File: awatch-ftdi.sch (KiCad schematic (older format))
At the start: 43 parts, among them J801 Molex 1050170001, J802 Conn_01x06, U801 AT93C46DN-SH-T, U802 MCP1703A-3302_SOT223, U803 FT2232HL, Y801 FH1200004

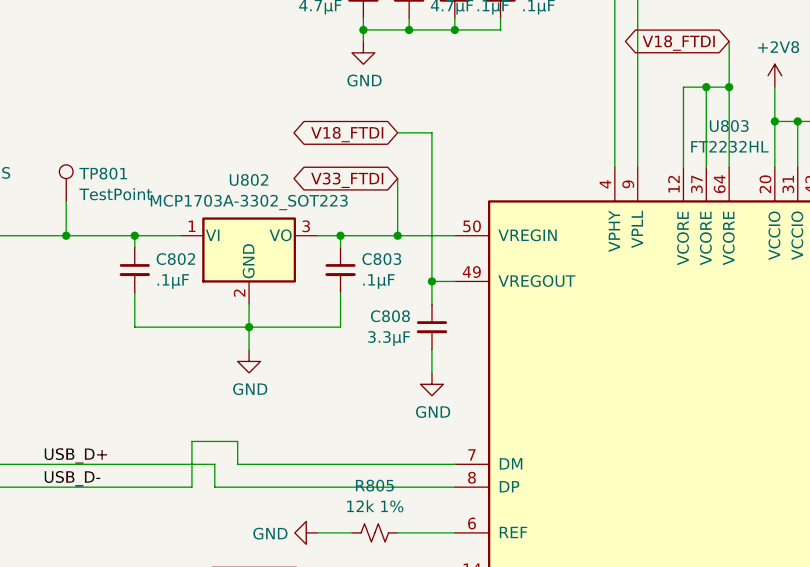
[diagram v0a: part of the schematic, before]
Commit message: Route FTDI.
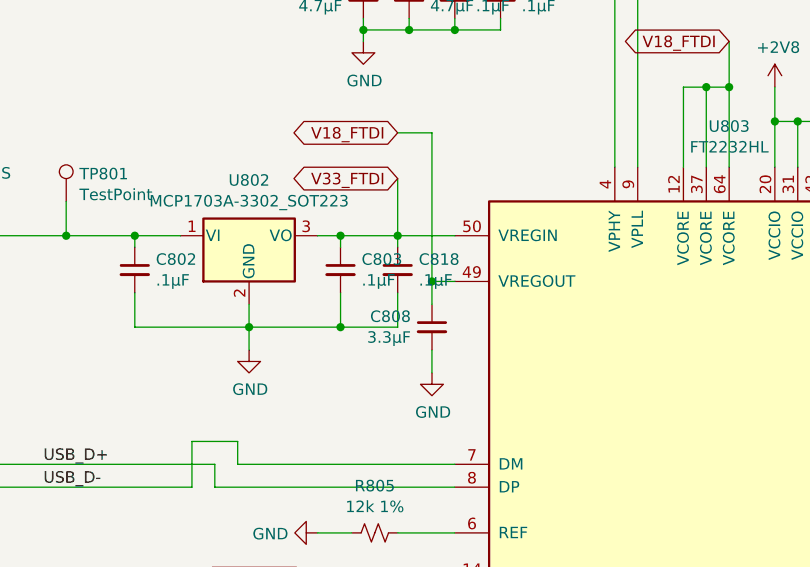
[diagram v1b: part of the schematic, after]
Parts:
- added C818: .1µF, Capacitor_SMD:C_0603_1608Metric, symbol Device:C_Small
- J802: footprint Connector_PinSocket_2.54mm:PinSocket_1x06_P2.54mm_Vertical -> Connector_PinHeader_2.54mm:PinHeader_1x06_P2.54mm_Vertical
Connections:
- net GND: now also C818.2
- net V33_FTDI: now also C818.1
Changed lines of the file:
@@
 F 0 "J802" H 10280 2792 50  0000 L CNN
 F 1 "Conn_01x06" H 10280 2701 50  0000 L CNN
-F 2 "Connector_PinSocket_2.54mm:PinSocket_1x06_P2.54mm_Vertical" H 10200 2800 50  0001 C CNN
+F 2 "Connector_PinHeader_2.54mm:PinHeader_1x06_P2.54mm_Vertical" H 10200 2800 50  0001 C CNN
 F 3 "~" H 10200 2800 50  0001 C CNN
 	1    10200 2800
@@
 Wire Wire Line
 	2500 3350 2500 2550
-Wire Wire Line
-	2500 2550 2850 2550
 Connection ~ 3150 2550
 $Comp
@@
 	2850 2400 2850 2550
 Connection ~ 2850 2550
-Wire Wire Line
-	2850 2550 3150 2550
 $Comp
 L Device:C_Small C804
@@
 Text Label 2650 5450 0    50   ~ 0
 DO
+Wire Wire Line
+	2850 2550 3150 2550
+Wire Wire Line
+	2500 2550 2850 2550
+$Comp
+L Device:C_Small C818
+U 1 1 5C2F6C15
+P 4300 2700
+F 0 "C818" H 4392 2746 50  0000 L CNN
+F 1 ".1µF" H 4392 2655 50  0000 L CNN
+F 2 "Capacitor_SMD:C_0603_1608Metric" H 4300 2700 50  0001 C CNN
+F 3 "~" H 4300 2700 50  0001 C CNN
+	1    4300 2700
+	1    0    0    -1
+$EndComp
+Wire Wire Line
+	4300 2550 4300 2600
+Wire Wire Line
+	4300 2800 4300 2950
+Wire Wire Line
+	4300 2950 4050 2950
+Connection ~ 4050 2950
 $EndSCHEMATC

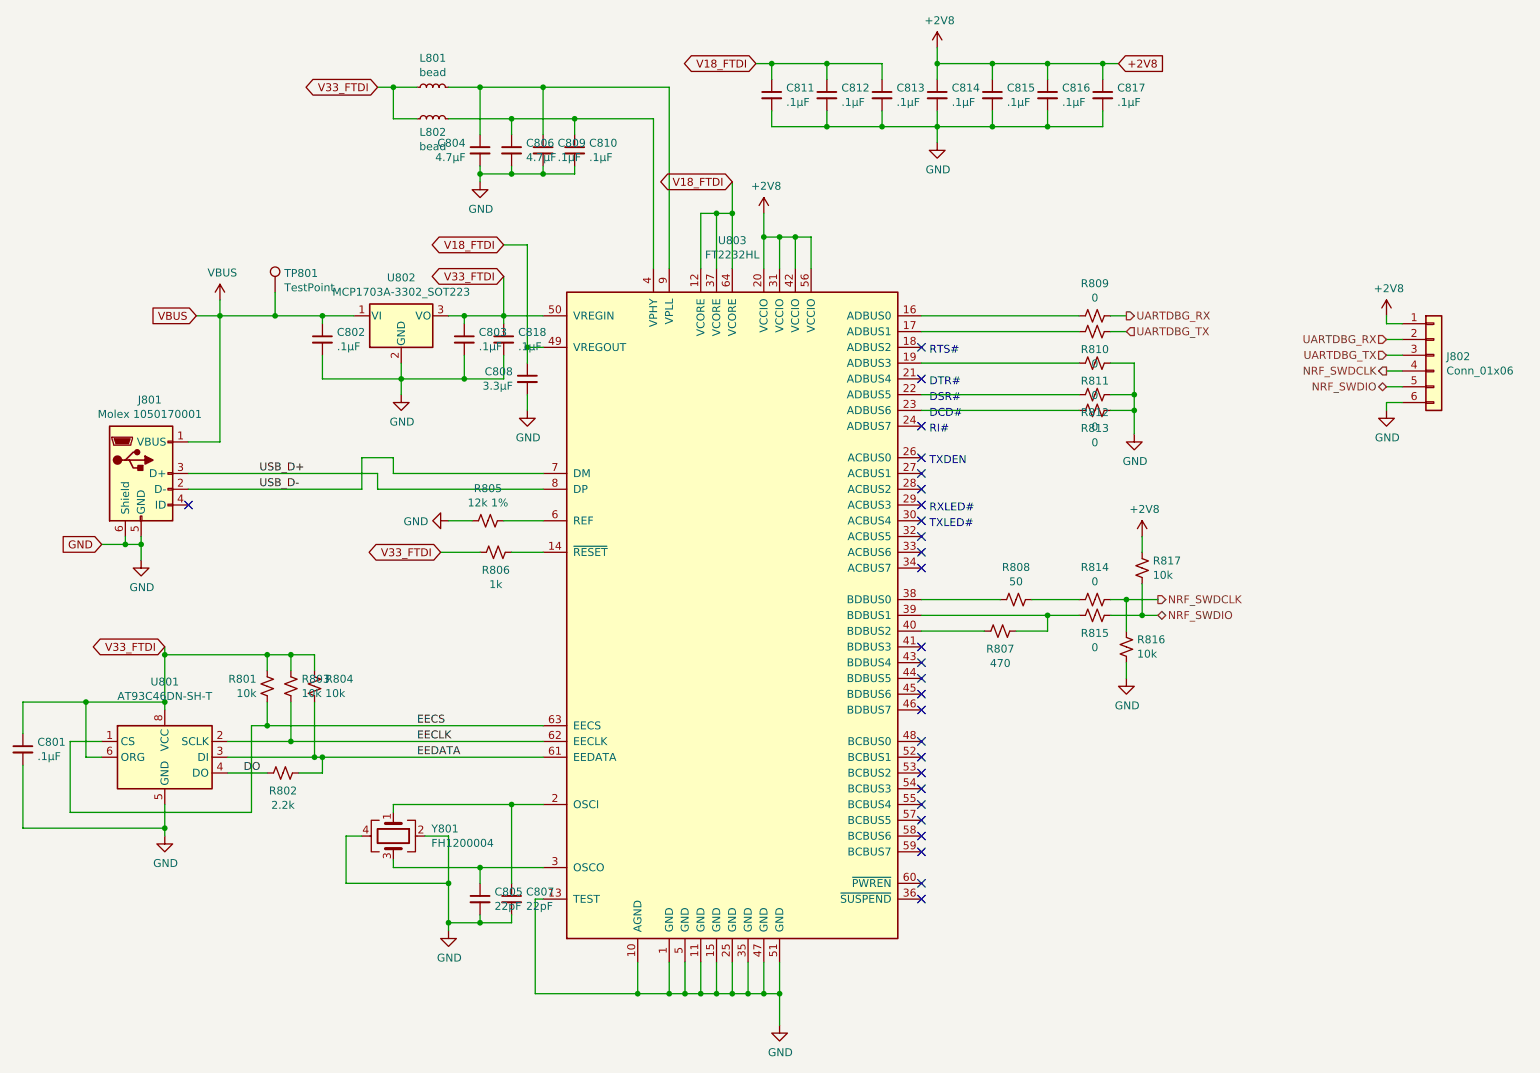
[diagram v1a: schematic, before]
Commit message: approx. final layout
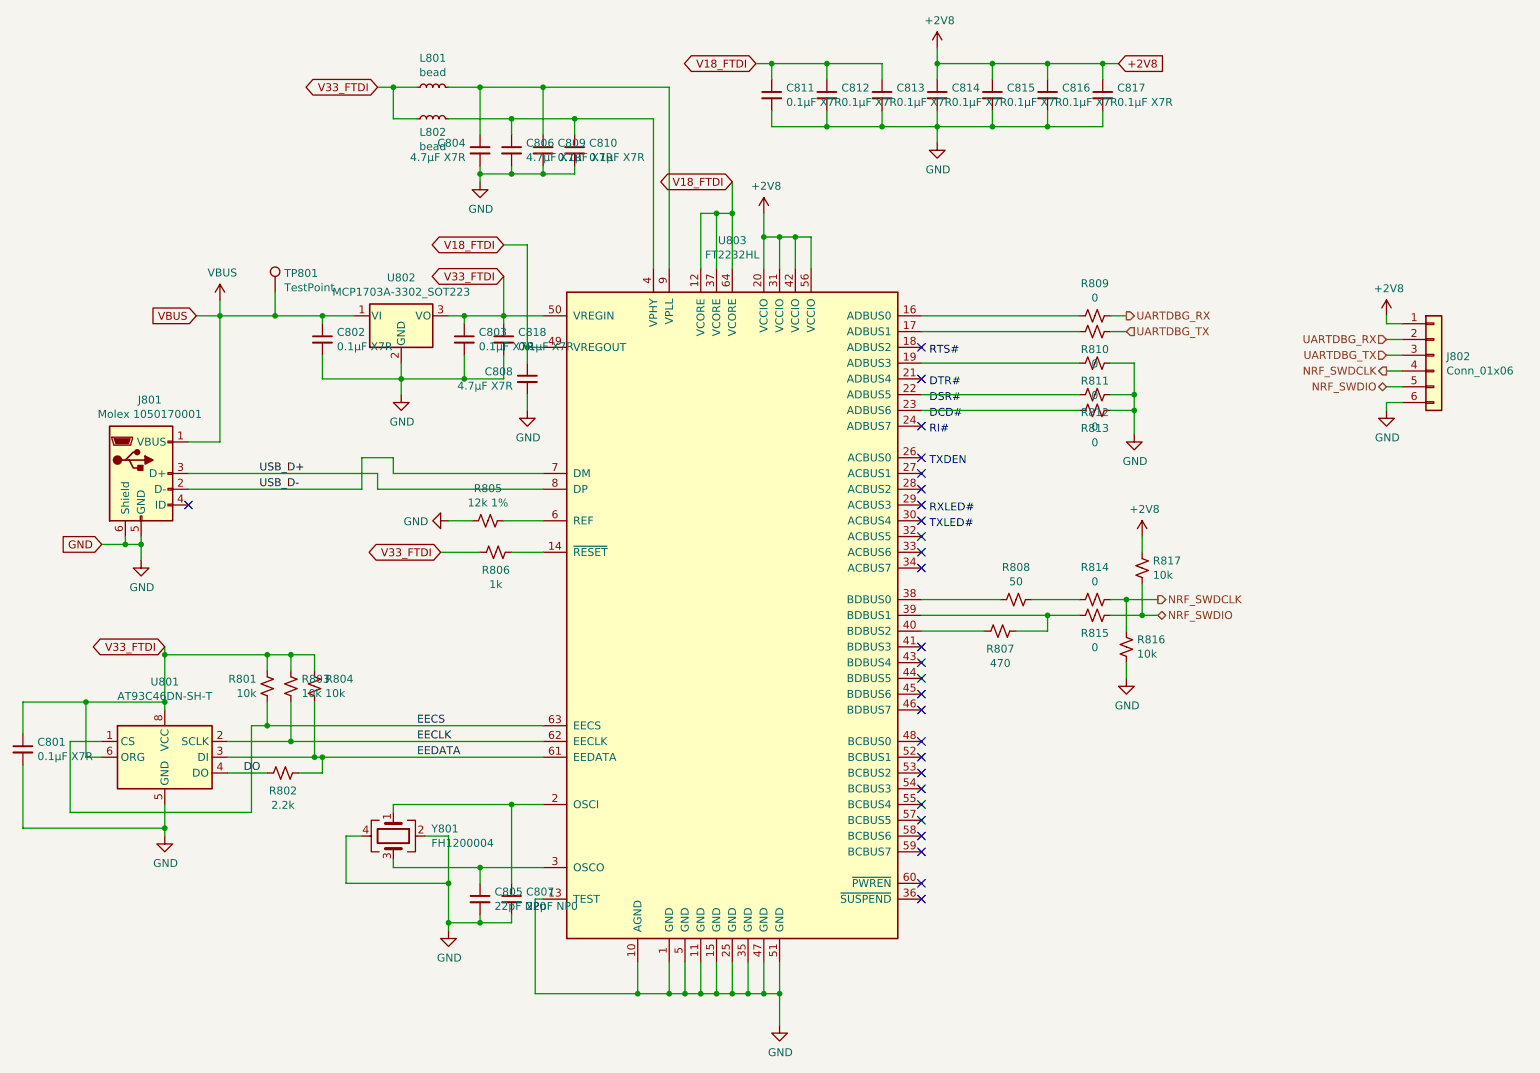
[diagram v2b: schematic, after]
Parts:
- C801, C802, C803, C809, C810, C811, C812, C813, C814, C815, C816, C817, C818: value .1µF -> 0.1µF X7R; DigiKey PN (none) -> 1276-1061-1-ND
- C804, C806: value 4.7µF -> 4.7µF X7R; DigiKey PN (none) -> 1276-2087-1-ND
- C805, C807: value 22pF -> 22pF NP0; DigiKey PN (none) -> 399-7874-1-ND
- C808: value 3.3µF -> 4.7µF X7R; DigiKey PN (none) -> 1276-2087-1-ND
- J801: DigiKey PN (none) -> WM1399CT-ND
- U801: DigiKey PN (none) -> AT93C46DN-SH-TCT-ND AT93C46DN-SH-TCT-ND
- U802: DigiKey PN (none) -> MCP1703AT-3302E/DBCT-ND
- U803: DigiKey PN (none) -> 768-1024-1-ND
- Y801: DigiKey PN (none) -> FH1200004CT-ND
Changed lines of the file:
@@
 $Descr A4 11693 8268
 encoding utf-8
-Sheet 8 9
+Sheet 8 10
 Title "AWatch2"
 Date ""
@@
 F 2 "Package_QFP:LQFP-64_10x10mm_P0.5mm" H 5750 4450 50  0001 C CNN
 F 3 "http://www.ftdichip.com/Products/ICs/FT2232H.html" H 5750 4450 50  0001 C CNN
+F 4 "768-1024-1-ND" H 0   0   50  0001 C CNN "DigiKey PN"
 	1    5750 4450
 	1    0    0    -1
@@
 F 2 "Package_TO_SOT_SMD:SOT-223-3_TabPin2" H 3650 2750 50  0001 C CNN
 F 3 "http://ww1.microchip.com/downloads/en/DeviceDoc/20005122B.pdf" H 3650 2500 50  0001 C CNN
+F 4 "MCP1703AT-3302E/DBCT-ND" H 0   0   50  0001 C CNN "DigiKey PN"
 	1    3650 2550
 	1    0    0    -1
@@
 F 2 "Package_SO:SOIC-8_3.9x4.9mm_P1.27mm" H 2150 5350 50  0001 C CNN
 F 3 "http://ww1.microchip.com/downloads/en/DeviceDoc/20001749K.pdf" H 2150 5350 50  0001 C CNN
+F 4 "AT93C46DN-SH-TCT-NDAT93C46DN-SH-TCT-ND" H 0   0   50  0001 C CNN "DigiKey PN"
 	1    2150 5350
 	1    0    0    -1
@@
 P 1250 5300
 F 0 "C801" H 1342 5346 50  0000 L CNN
-F 1 ".1µF" H 1342 5255 50  0000 L CNN
+F 1 "0.1µF X7R" H 1342 5255 50  0000 L CNN
 F 2 "Capacitor_SMD:C_0603_1608Metric" H 1250 5300 50  0001 C CNN
 F 3 "~" H 1250 5300 50  0001 C CNN
+F 4 "1276-1061-1-ND" H 0   0   50  0001 C CNN "DigiKey PN"
 	1    1250 5300
 	1    0    0    -1
@@
 P 4050 2700
 F 0 "C803" H 4142 2746 50  0000 L CNN
-F 1 ".1µF" H 4142 2655 50  0000 L CNN
+F 1 "0.1µF X7R" H 4142 2655 50  0000 L CNN
 F 2 "Capacitor_SMD:C_0603_1608Metric" H 4050 2700 50  0001 C CNN
 F 3 "~" H 4050 2700 50  0001 C CNN
+F 4 "1276-1061-1-ND" H 0   0   50  0001 C CNN "DigiKey PN"
 	1    4050 2700
 	1    0    0    -1
@@
 P 3150 2700
 F 0 "C802" H 3242 2746 50  0000 L CNN
-F 1 ".1µF" H 3242 2655 50  0000 L CNN
+F 1 "0.1µF X7R" H 3242 2655 50  0000 L CNN
 F 2 "Capacitor_SMD:C_0603_1608Metric" H 3150 2700 50  0001 C CNN
 F 3 "~" H 3150 2700 50  0001 C CNN
+F 4 "1276-1061-1-ND" H 0   0   50  0001 C CNN "DigiKey PN"
 	1    3150 2700
 	1    0    0    -1
@@
 P 4450 2950
 F 0 "C808" H 4358 2996 50  0000 R CNN
-F 1 "3.3µF" H 4358 2905 50  0000 R CNN
+F 1 "4.7µF X7R" H 4358 2905 50  0000 R CNN
 F 2 "Capacitor_SMD:C_0603_1608Metric" H 4450 2950 50  0001 C CNN
 F 3 "~" H 4450 2950 50  0001 C CNN
+F 4 "1276-2087-1-ND" H 0   0   50  0001 C CNN "DigiKey PN"
 	1    4450 2950
 	1    0    0    -1
@@
 P 4550 1500
 F 0 "C809" H 4642 1546 50  0000 L CNN
-F 1 ".1µF" H 4642 1455 50  0000 L CNN
+F 1 "0.1µF X7R" H 4642 1455 50  0000 L CNN
 F 2 "Capacitor_SMD:C_0603_1608Metric" H 4550 1500 50  0001 C CNN
 F 3 "~" H 4550 1500 50  0001 C CNN
+F 4 "1276-1061-1-ND" H 0   0   50  0001 C CNN "DigiKey PN"
 	1    4550 1500
 	1    0    0    -1
@@
 P 4750 1500
 F 0 "C810" H 4842 1546 50  0000 L CNN
-F 1 ".1µF" H 4842 1455 50  0000 L CNN
+F 1 "0.1µF X7R" H 4842 1455 50  0000 L CNN
 F 2 "Capacitor_SMD:C_0603_1608Metric" H 4750 1500 50  0001 C CNN
 F 3 "~" H 4750 1500 50  0001 C CNN
+F 4 "1276-1061-1-ND" H 0   0   50  0001 C CNN "DigiKey PN"
 	1    4750 1500
 	1    0    0    -1
@@
 P 6000 1150
 F 0 "C811" H 6092 1196 50  0000 L CNN
-F 1 ".1µF" H 6092 1105 50  0000 L CNN
+F 1 "0.1µF X7R" H 6092 1105 50  0000 L CNN
 F 2 "Capacitor_SMD:C_0603_1608Metric" H 6000 1150 50  0001 C CNN
 F 3 "~" H 6000 1150 50  0001 C CNN
+F 4 "1276-1061-1-ND" H 0   0   50  0001 C CNN "DigiKey PN"
 	1    6000 1150
 	1    0    0    -1
@@
 P 6350 1150
 F 0 "C812" H 6442 1196 50  0000 L CNN
-F 1 ".1µF" H 6442 1105 50  0000 L CNN
+F 1 "0.1µF X7R" H 6442 1105 50  0000 L CNN
 F 2 "Capacitor_SMD:C_0603_1608Metric" H 6350 1150 50  0001 C CNN
 F 3 "~" H 6350 1150 50  0001 C CNN
+F 4 "1276-1061-1-ND" H 0   0   50  0001 C CNN "DigiKey PN"
 	1    6350 1150
 	1    0    0    -1
@@
 P 6700 1150
 F 0 "C813" H 6792 1196 50  0000 L CNN
-F 1 ".1µF" H 6792 1105 50  0000 L CNN
+F 1 "0.1µF X7R" H 6792 1105 50  0000 L CNN
 F 2 "Capacitor_SMD:C_0603_1608Metric" H 6700 1150 50  0001 C CNN
 F 3 "~" H 6700 1150 50  0001 C CNN
+F 4 "1276-1061-1-ND" H 0   0   50  0001 C CNN "DigiKey PN"
 	1    6700 1150
 	1    0    0    -1
@@
 P 7050 1150
 F 0 "C814" H 7142 1196 50  0000 L CNN
-F 1 ".1µF" H 7142 1105 50  0000 L CNN
+F 1 "0.1µF X7R" H 7142 1105 50  0000 L CNN
 F 2 "Capacitor_SMD:C_0603_1608Metric" H 7050 1150 50  0001 C CNN
 F 3 "~" H 7050 1150 50  0001 C CNN
+F 4 "1276-1061-1-ND" H 0   0   50  0001 C CNN "DigiKey PN"
 	1    7050 1150
 	1    0    0    -1
@@
 P 7400 1150
 F 0 "C815" H 7492 1196 50  0000 L CNN
-F 1 ".1µF" H 7492 1105 50  0000 L CNN
+F 1 "0.1µF X7R" H 7492 1105 50  0000 L CNN
 F 2 "Capacitor_SMD:C_0603_1608Metric" H 7400 1150 50  0001 C CNN
 F 3 "~" H 7400 1150 50  0001 C CNN
+F 4 "1276-1061-1-ND" H 0   0   50  0001 C CNN "DigiKey PN"
 	1    7400 1150
 	1    0    0    -1
@@
 P 7750 1150
 F 0 "C816" H 7842 1196 50  0000 L CNN
-F 1 ".1µF" H 7842 1105 50  0000 L CNN
+F 1 "0.1µF X7R" H 7842 1105 50  0000 L CNN
 F 2 "Capacitor_SMD:C_0603_1608Metric" H 7750 1150 50  0001 C CNN
 F 3 "~" H 7750 1150 50  0001 C CNN
+F 4 "1276-1061-1-ND" H 0   0   50  0001 C CNN "DigiKey PN"
 	1    7750 1150
 	1    0    0    -1
@@
 P 8100 1150
 F 0 "C817" H 8192 1196 50  0000 L CNN
-F 1 ".1µF" H 8192 1105 50  0000 L CNN
+F 1 "0.1µF X7R" H 8192 1105 50  0000 L CNN
 F 2 "Capacitor_SMD:C_0603_1608Metric" H 8100 1150 50  0001 C CNN
 F 3 "~" H 8100 1150 50  0001 C CNN
+F 4 "1276-1061-1-ND" H 0   0   50  0001 C CNN "DigiKey PN"
 	1    8100 1150
 	1    0    0    -1
@@
 F 2 "Crystal:Crystal_SMD_2520-4Pin_2.5x2.0mm" H 3600 5850 50  0001 C CNN
 F 3 "~" H 3600 5850 50  0001 C CNN
+F 4 "FH1200004CT-ND" H 0   0   50  0001 C CNN "DigiKey PN"
 	1    3600 5850
 	0    1    1    0
@@
 P 4150 6250
 F 0 "C805" H 4242 6296 50  0000 L CNN
-F 1 "22pF" H 4242 6205 50  0000 L CNN
+F 1 "22pF NP0" H 4242 6205 50  0000 L CNN
 F 2 "Capacitor_SMD:C_0603_1608Metric" H 4150 6250 50  0001 C CNN
 F 3 "~" H 4150 6250 50  0001 C CNN
+F 4 "399-7874-1-ND" H 0   0   50  0001 C CNN "DigiKey PN"
 	1    4150 6250
 	1    0    0    -1
@@
 P 4350 6250
 F 0 "C807" H 4442 6296 50  0000 L CNN
-F 1 "22pF" H 4442 6205 50  0000 L CNN
+F 1 "22pF NP0" H 4442 6205 50  0000 L CNN
 F 2 "Capacitor_SMD:C_0603_1608Metric" H 4350 6250 50  0001 C CNN
 F 3 "~" H 4350 6250 50  0001 C CNN
+F 4 "399-7874-1-ND" H 0   0   50  0001 C CNN "DigiKey PN"
 	1    4350 6250
 	1    0    0    -1
@@
 F 2 "Connector_USB:USB_Micro-B_Molex-105017-0001" H 2150 3500 50  0001 C CNN
 F 3 "~" H 2150 3500 50  0001 C CNN
+F 4 "WM1399CT-ND" H 0   0   50  0001 C CNN "DigiKey PN"
 	1    2000 3550
 	1    0    0    -1
@@
 P 4150 1500
 F 0 "C804" H 4242 1546 50  0000 L CNN
-F 1 "4.7µF" H 4242 1455 50  0000 L CNN
+F 1 "4.7µF X7R" H 4242 1455 50  0000 L CNN
 F 2 "Capacitor_SMD:C_0603_1608Metric" H 4150 1500 50  0001 C CNN
 F 3 "~" H 4150 1500 50  0001 C CNN
+F 4 "1276-2087-1-ND" H 0   0   50  0001 C CNN "DigiKey PN"
 	1    4150 1500
 	-1   0    0    -1
@@
 P 4350 1500
 F 0 "C806" H 4442 1546 50  0000 L CNN
-F 1 "4.7µF" H 4442 1455 50  0000 L CNN
+F 1 "4.7µF X7R" H 4442 1455 50  0000 L CNN
 F 2 "Capacitor_SMD:C_0603_1608Metric" H 4350 1500 50  0001 C CNN
 F 3 "~" H 4350 1500 50  0001 C CNN
+F 4 "1276-2087-1-ND" H 0   0   50  0001 C CNN "DigiKey PN"
 	1    4350 1500
 	1    0    0    -1
@@
 P 4300 2700
 F 0 "C818" H 4392 2746 50  0000 L CNN
-F 1 ".1µF" H 4392 2655 50  0000 L CNN
+F 1 "0.1µF X7R" H 4392 2655 50  0000 L CNN
 F 2 "Capacitor_SMD:C_0603_1608Metric" H 4300 2700 50  0001 C CNN
 F 3 "~" H 4300 2700 50  0001 C CNN
+F 4 "1276-1061-1-ND" H 0   0   50  0001 C CNN "DigiKey PN"
 	1    4300 2700
 	1    0    0    -1
